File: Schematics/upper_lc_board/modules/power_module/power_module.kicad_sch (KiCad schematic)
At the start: 29 parts, among them U3 LD1117S33TR_SOT223, U4 ID_LM66100DCKR, U5 ID_LM66100DCKR, U9 TVS3300DRV

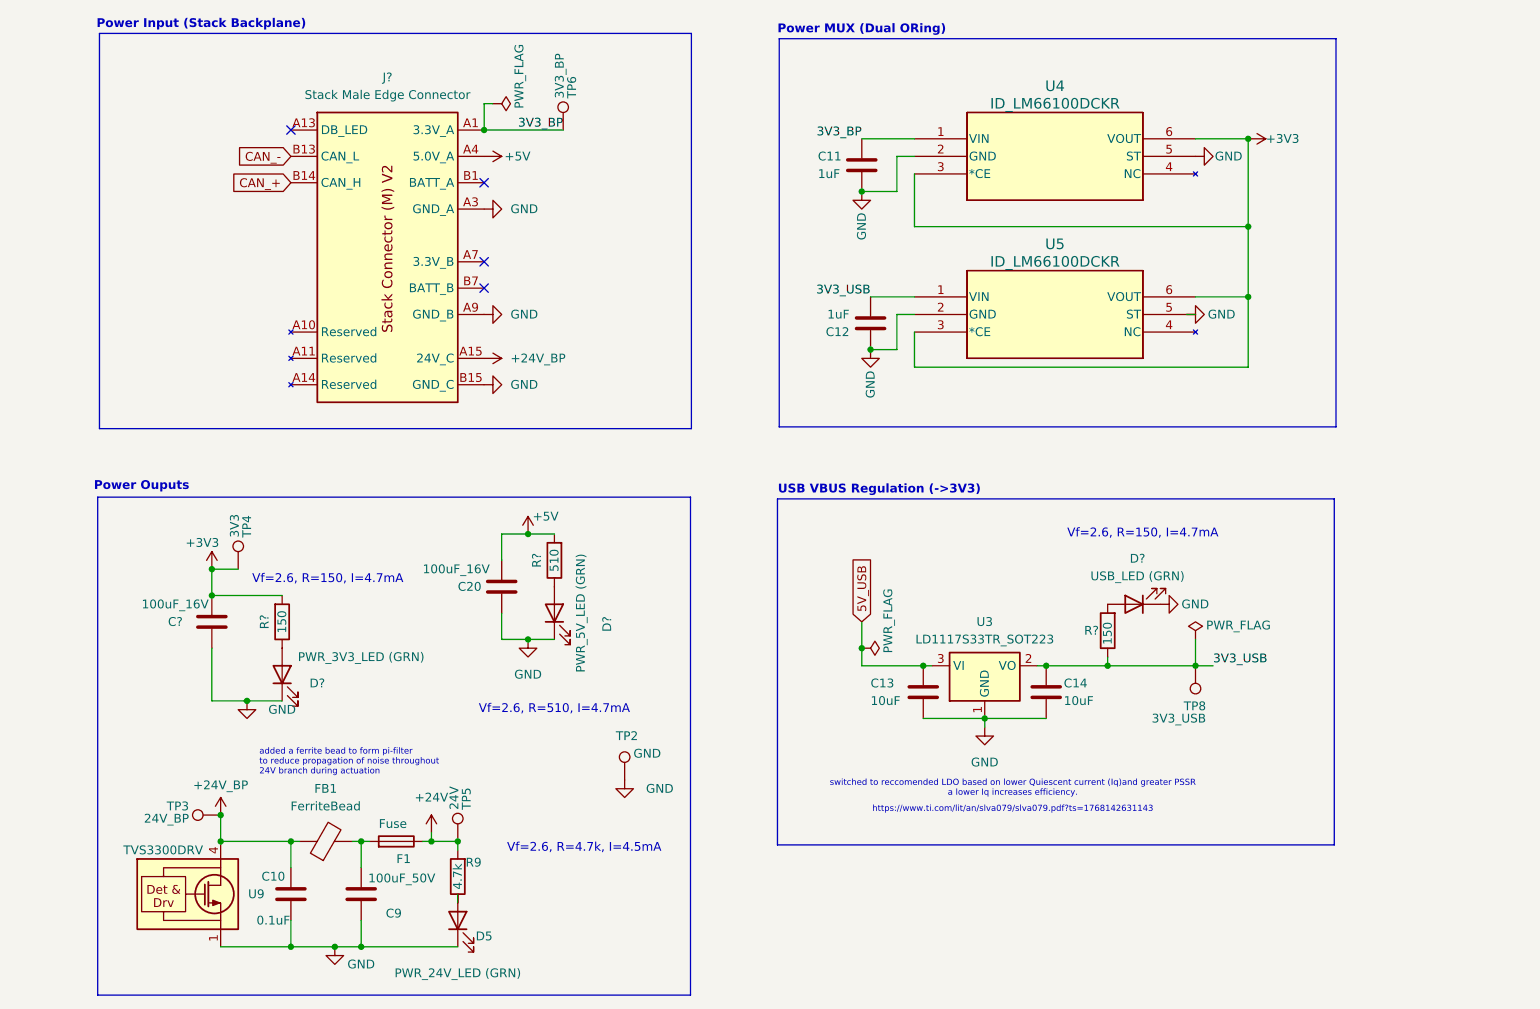
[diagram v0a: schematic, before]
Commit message: organizational work
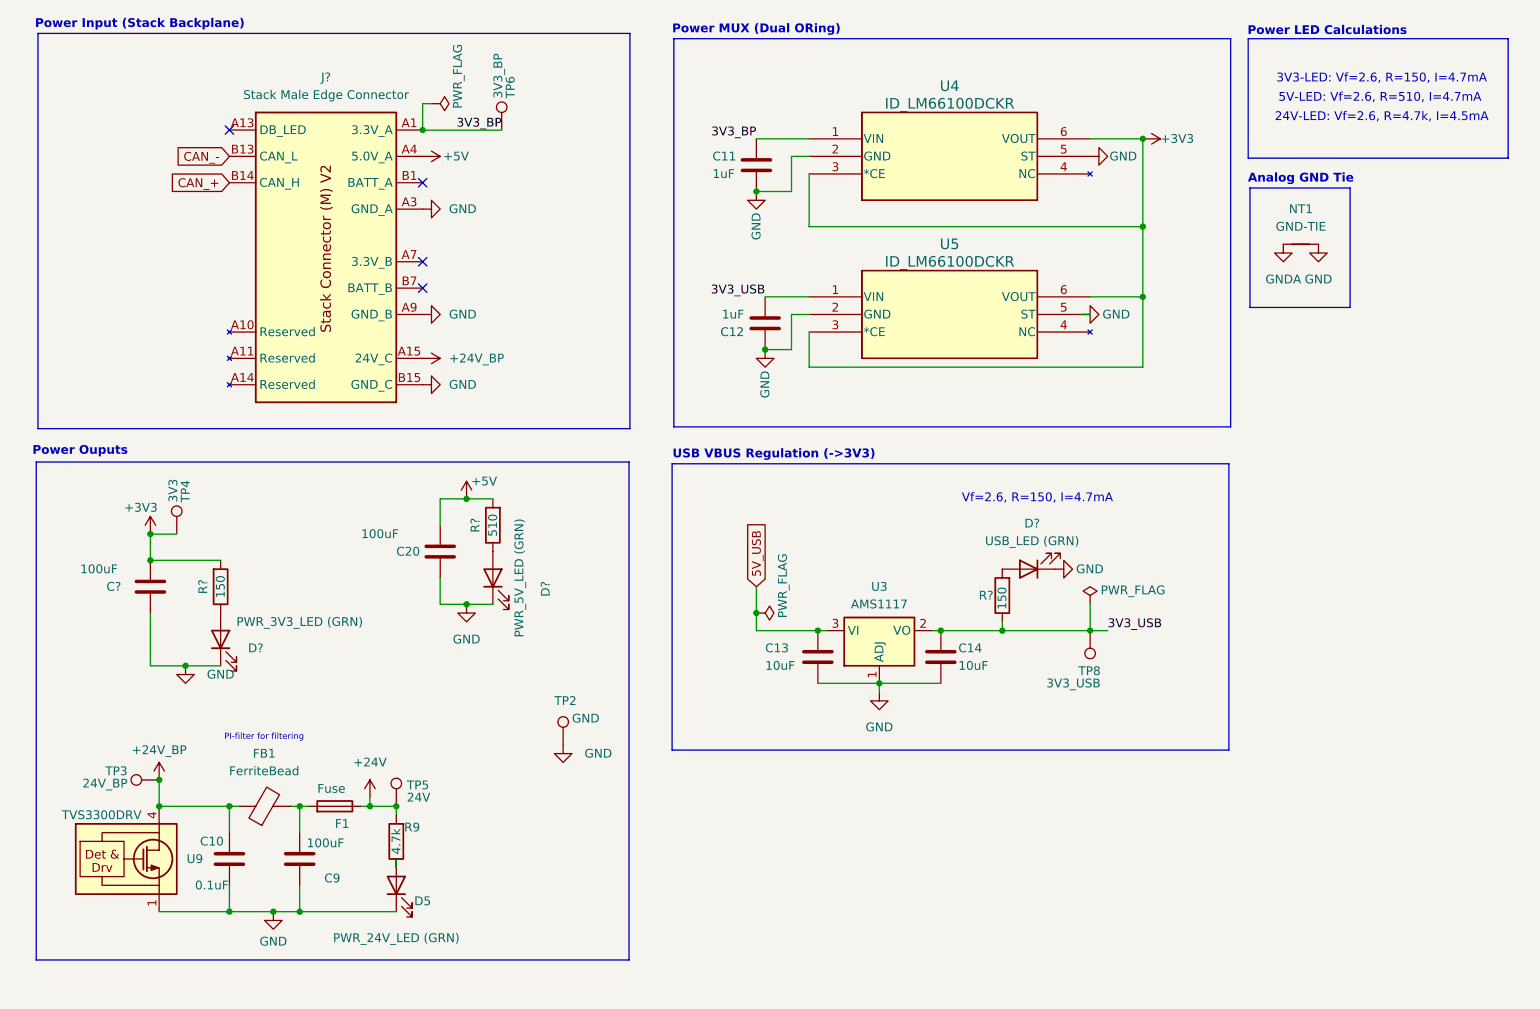
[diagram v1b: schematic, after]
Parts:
- added NT1: GND-TIE, NetTie:NetTie-2_SMD_Pad0.5mm, symbol Device:NetTie_2
- C10: JLCPCB (none) -> C14663
- C11, C12: JLCPCB (none) -> C15849
- C20, C?: value 100uF_16V -> 100uF
- C9: value 100uF_50V -> 100uF
- U3: value LD1117S33TR_SOT223 -> AMS1117; symbol Regulator_Linear:LD1117S33TR_SOT223 -> Regulator_Linear:AMS1117
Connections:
- net GND: now also NT1.2
- new net GNDA: NT1.1
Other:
- note added: "24V-LED: Vf=2.6, R=4.7k, I=4.5mA"
- note added: "3V3-LED: Vf=2.6, R=150, I=4.7mA"
- note added: "5V-LED: Vf=2.6, R=510, I=4.7mA"
- note added: "Analog GND Tie"
- note added: "PI-filter for filtering"
- note added: "Power LED Calculations"
- note removed: "Vf=2.6, R=4.7k, I=4.5mA"
- note removed: "Vf=2.6, R=510, I=4.7mA"
- note removed: "added a ferrite bead to form pi-filter to reduce propagation of noise throughout 24V branch during actuation"
- note removed: "https://www.ti.com/lit/an/slva079/slva079.pdf?ts=1768142631143"
- note removed: "switched to reccomended LDO based on lower Quiescent current (Iq)and greater PSSR a lower Iq increases efficiency."
- moved on the sheet: C10, C11, C12, C13, C14, C20, C9, C?, D5, D?, F1, FB1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
